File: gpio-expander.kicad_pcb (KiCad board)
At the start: 2 copper layers, 59 x 33.4 mm, 5 parts, among them U1 TPS4H160AQPWPRQ1, U2 TPS4H160AQPWPRQ1, U3 TPS4H160AQPWPRQ1, U4 TPS4H160AQPWPRQ1, U5 MCP23017T-E_SO

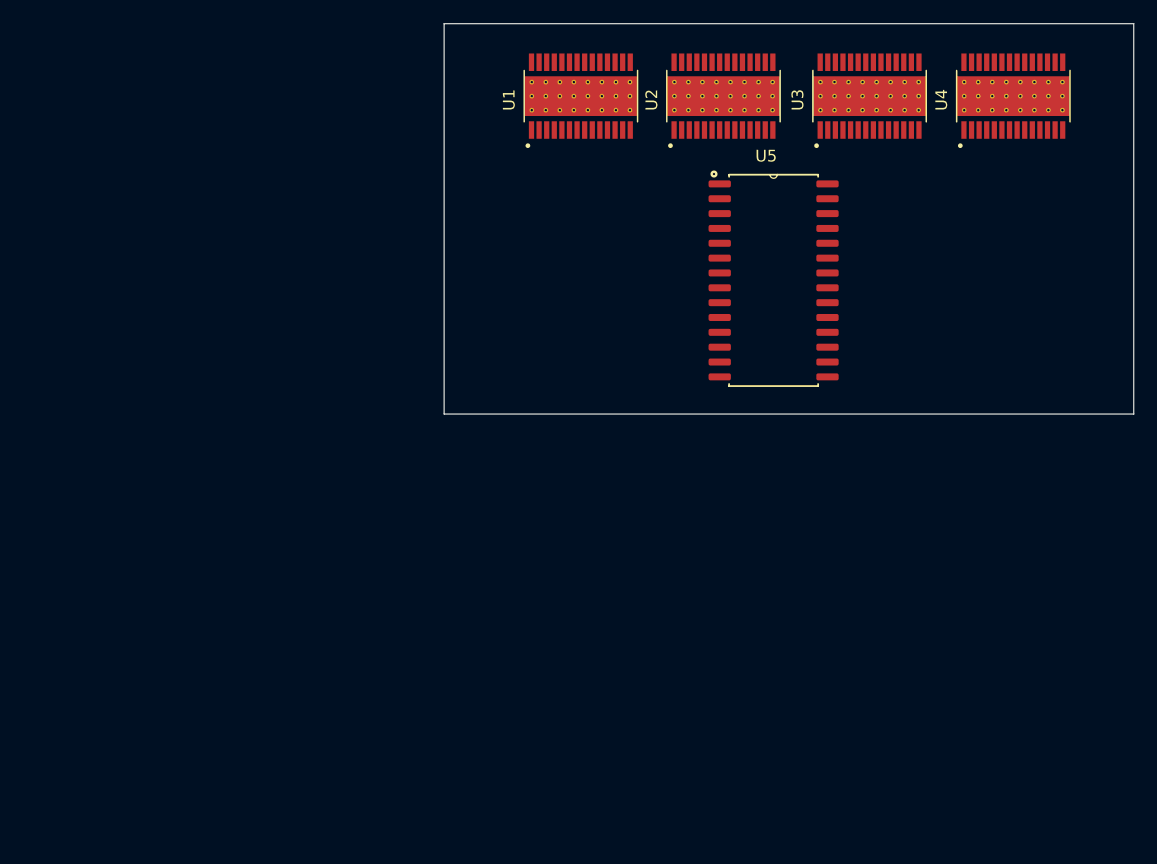
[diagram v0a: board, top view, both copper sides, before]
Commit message: first pcb revision
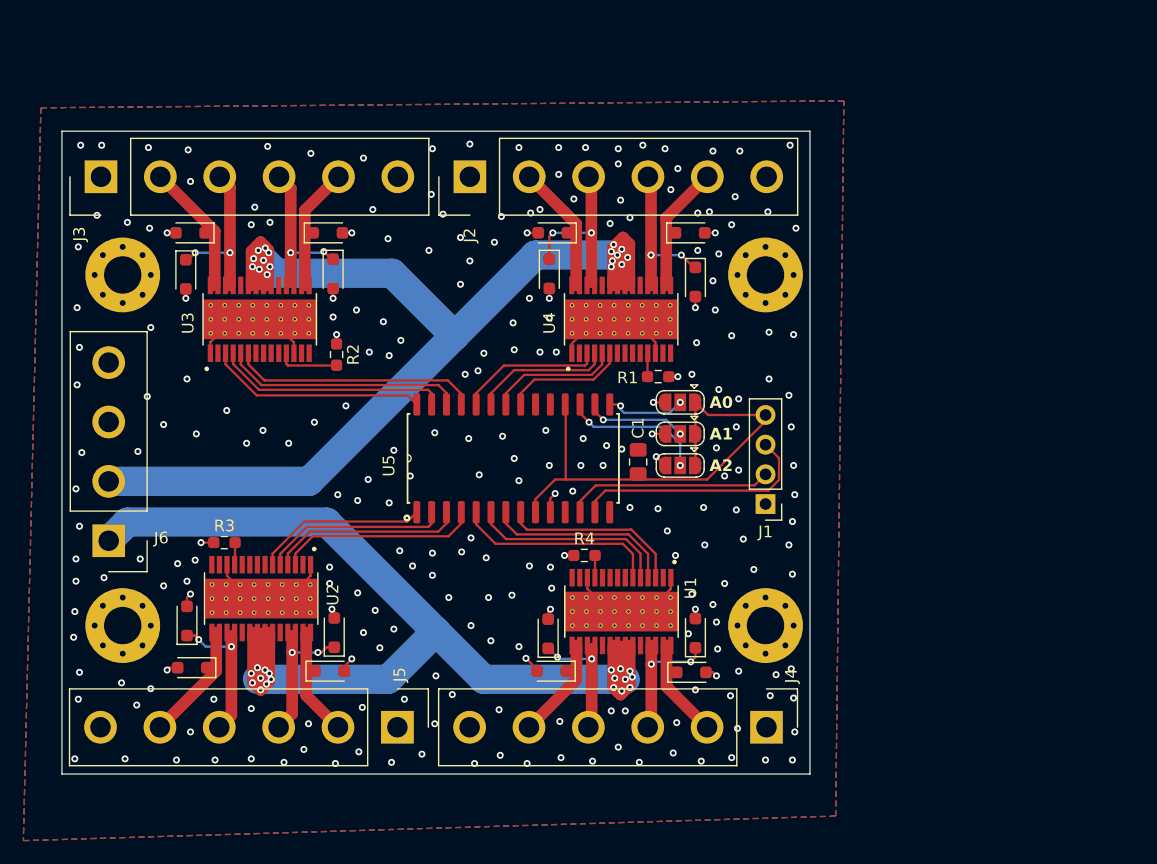
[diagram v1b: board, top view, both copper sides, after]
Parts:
- added C1: C, Capacitor_SMD:C_0805_2012Metric_Pad1.18x1.45mm_HandSolder, F.Cu at (119.1, 81.0)
- added D1: 60V 1A, Diode_SMD:D_SOD-323_HandSoldering, F.Cu at (80.8, 61.4)
- added D10: 60V 1A, Diode_SMD:D_SOD-323_HandSoldering, F.Cu at (124.0, 95.7)
- added D11: 60V 1A, Diode_SMD:D_SOD-323_HandSoldering, F.Cu at (111.4, 95.7)
- added D12: 60V 1A, Diode_SMD:D_SOD-323_HandSoldering, F.Cu at (111.7, 98.9)
- added D13: 60V 1A, Diode_SMD:D_SOD-323_HandSoldering, F.Cu at (92.7, 98.9)
- added D14: 60V 1A, Diode_SMD:D_SOD-323_HandSoldering, F.Cu at (93.1, 95.6)
- added D15: 60V 1A, Diode_SMD:D_SOD-323_HandSoldering, F.Cu at (80.5, 94.6)
- added D16: 60V 1A, Diode_SMD:D_SOD-323_HandSoldering, F.Cu at (81.0, 98.6)
- added D2: 60V 1A, Diode_SMD:D_SOD-323_HandSoldering, F.Cu at (80.4, 65.0)
- added D3: 60V 1A, Diode_SMD:D_SOD-323_HandSoldering, F.Cu at (93.0, 64.9)
- added D4: 60V 1A, Diode_SMD:D_SOD-323_HandSoldering, F.Cu at (92.5, 61.4)
- added D5: 60V 1A, Diode_SMD:D_SOD-323_HandSoldering, F.Cu at (123.5, 61.4)
- added D6: 60V 1A, Diode_SMD:D_SOD-323_HandSoldering, F.Cu at (124.0, 65.6)
- added D7: 60V 1A, Diode_SMD:D_SOD-323_HandSoldering, F.Cu at (111.5, 64.9)
- added D8: 60V 1A, Diode_SMD:D_SOD-323_HandSoldering, F.Cu at (111.8, 61.4)
- added D9: 60V 1A, Diode_SMD:D_SOD-323_HandSoldering, F.Cu at (123.7, 99.0)
- added H1: MountingHole_Pad, MountingHole:MountingHole_3.2mm_M3_Pad_Via, F.Cu at (75.0, 65.0)
- added H2: MountingHole_Pad, MountingHole:MountingHole_3.2mm_M3_Pad_Via, F.Cu at (130.0, 65.0)
- added H3: MountingHole_Pad, MountingHole:MountingHole_3.2mm_M3_Pad_Via, F.Cu at (130.0, 95.0)
- added H4: MountingHole_Pad, MountingHole:MountingHole_3.2mm_M3_Pad_Via, F.Cu at (75.0, 95.0)
- added J1: Conn_01x04, Connector_PinHeader_2.54mm:PinHeader_1x04_P2.54mm_Vertical, F.Cu at (130.0, 84.6)
- added J2: Conn_01x06, Connector_Samtec_HPM_THT:Samtec_HPM-06-05-x-S_Straight_1x06_Pitch5.08mm, F.Cu at (104.7, 56.6)
- added J3: Conn_01x06, Connector_Samtec_HPM_THT:Samtec_HPM-06-05-x-S_Straight_1x06_Pitch5.08mm, F.Cu at (73.1, 56.6)
- added J4: Conn_01x06, Connector_Samtec_HPM_THT:Samtec_HPM-06-05-x-S_Straight_1x06_Pitch5.08mm, F.Cu at (130.1, 103.7)
- added J5: Conn_01x06, Connector_Samtec_HPM_THT:Samtec_HPM-06-05-x-S_Straight_1x06_Pitch5.08mm, F.Cu at (98.5, 103.7)
- added J6: Conn_01x04, Connector_Samtec_HPM_THT:Samtec_HPM-04-05-x-S_Straight_1x04_Pitch5.08mm, F.Cu at (73.8, 87.7)
- added JP1: SolderJumper_3_Open, Jumper:SolderJumper-3_P1.3mm_Open_RoundedPad1.0x1.5mm, F.Cu at (122.7, 75.9)
- added JP2: SolderJumper_3_Open, Jumper:SolderJumper-3_P1.3mm_Open_RoundedPad1.0x1.5mm, F.Cu at (122.7, 78.6)
- added JP3: SolderJumper_3_Open, Jumper:SolderJumper-3_P1.3mm_Open_RoundedPad1.0x1.5mm, F.Cu at (122.7, 81.3)
- added R1: R, Resistor_SMD:R_0603_1608Metric_Pad0.98x0.95mm_HandSolder, F.Cu at (120.8, 73.7)
- added R2: R, Resistor_SMD:R_0603_1608Metric_Pad0.98x0.95mm_HandSolder, F.Cu at (93.3, 71.8)
- added R3: R, Resistor_SMD:R_0603_1608Metric_Pad0.98x0.95mm_HandSolder, F.Cu at (83.7, 87.9)
- added R4: R, Resistor_SMD:R_0603_1608Metric_Pad0.98x0.95mm_HandSolder, F.Cu at (114.5, 89.0)
- moved U2 58.4 mm to (86.8, 92.7), turned to -90 degrees
- moved U3 55.6 mm to (86.7, 68.8)
- moved U1 44.2 mm to (117.7, 93.8), turned to -90 degrees
- moved U4 38.6 mm to (117.7, 68.8)
- moved U5 27.0 mm to (108.4, 80.7), turned to 90 degrees
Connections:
- U1 pad 1: Net-(U1-GND-Pad1) -> GND
- U1 pad 11: unconnected-(U1-CL-Pad11) -> Net-(U1-CL)
- U1 pad 12: Net-(U1-GND-Pad1) -> GND
- U1 pad 20: Net-(U1-VS-Pad20) -> +24V
- U1 pad 21: Net-(U1-VS-Pad20) -> +24V
- U1 pad 22: Net-(U1-VS-Pad20) -> +24V
- U1 pad 23: Net-(U1-VS-Pad20) -> +24V
- U1 pad 29: Net-(U1-EXP-Pad29) -> GND
- U1 pad 30: Net-(U1-EXP-Pad29) -> GND
- U1 pad 31: Net-(U1-EXP-Pad29) -> GND
- U1 pad 32: Net-(U1-EXP-Pad29) -> GND
- U1 pad 33: Net-(U1-EXP-Pad29) -> GND
- U1 pad 34: Net-(U1-EXP-Pad29) -> GND
- U1 pad 35: Net-(U1-EXP-Pad29) -> GND
- U1 pad 36: Net-(U1-EXP-Pad29) -> GND
- U1 pad 37: Net-(U1-EXP-Pad29) -> GND
- U1 pad 38: Net-(U1-EXP-Pad29) -> GND
- U1 pad 39: Net-(U1-EXP-Pad29) -> GND
- U1 pad 40: Net-(U1-EXP-Pad29) -> GND
- U1 pad 41: Net-(U1-EXP-Pad29) -> GND
- U1 pad 42: Net-(U1-EXP-Pad29) -> GND
- U1 pad 43: Net-(U1-EXP-Pad29) -> GND
- U1 pad 44: Net-(U1-EXP-Pad29) -> GND
- U1 pad 45: Net-(U1-EXP-Pad29) -> GND
- U1 pad 46: Net-(U1-EXP-Pad29) -> GND
- U1 pad 47: Net-(U1-EXP-Pad29) -> GND
- U1 pad 48: Net-(U1-EXP-Pad29) -> GND
- U1 pad 49: Net-(U1-EXP-Pad29) -> GND
- U1 pad 50: Net-(U1-EXP-Pad29) -> GND
- U1 pad 51: Net-(U1-EXP-Pad29) -> GND
- U1 pad 52: Net-(U1-EXP-Pad29) -> GND
- U1 pad 53: Net-(U1-EXP-Pad29) -> GND
- U2 pad 1: Net-(U2-GND-Pad1) -> GND
- U2 pad 11: unconnected-(U2-CL-Pad11) -> Net-(U2-CL)
- U2 pad 12: Net-(U2-GND-Pad1) -> GND
- U2 pad 20: Net-(U2-VS-Pad20) -> +24V
- U2 pad 21: Net-(U2-VS-Pad20) -> +24V
- U2 pad 22: Net-(U2-VS-Pad20) -> +24V
- U2 pad 23: Net-(U2-VS-Pad20) -> +24V
- U2 pad 29: Net-(U2-EXP-Pad29) -> GND
- U2 pad 30: Net-(U2-EXP-Pad29) -> GND
- U2 pad 31: Net-(U2-EXP-Pad29) -> GND
- U2 pad 32: Net-(U2-EXP-Pad29) -> GND
- U2 pad 33: Net-(U2-EXP-Pad29) -> GND
- U2 pad 34: Net-(U2-EXP-Pad29) -> GND
- U2 pad 35: Net-(U2-EXP-Pad29) -> GND
- U2 pad 36: Net-(U2-EXP-Pad29) -> GND
- U2 pad 37: Net-(U2-EXP-Pad29) -> GND
- U2 pad 38: Net-(U2-EXP-Pad29) -> GND
- U2 pad 39: Net-(U2-EXP-Pad29) -> GND
- U2 pad 40: Net-(U2-EXP-Pad29) -> GND
- U2 pad 41: Net-(U2-EXP-Pad29) -> GND
- U2 pad 42: Net-(U2-EXP-Pad29) -> GND
- U2 pad 43: Net-(U2-EXP-Pad29) -> GND
- U2 pad 44: Net-(U2-EXP-Pad29) -> GND
- U2 pad 45: Net-(U2-EXP-Pad29) -> GND
- U2 pad 46: Net-(U2-EXP-Pad29) -> GND
- U2 pad 47: Net-(U2-EXP-Pad29) -> GND
- U2 pad 48: Net-(U2-EXP-Pad29) -> GND
- U2 pad 49: Net-(U2-EXP-Pad29) -> GND
- U2 pad 50: Net-(U2-EXP-Pad29) -> GND
- U2 pad 51: Net-(U2-EXP-Pad29) -> GND
- U2 pad 52: Net-(U2-EXP-Pad29) -> GND
- U2 pad 53: Net-(U2-EXP-Pad29) -> GND
- U3 pad 1: Net-(U3-GND-Pad1) -> GND
- U3 pad 11: unconnected-(U3-CL-Pad11) -> Net-(U3-CL)
- U3 pad 12: Net-(U3-GND-Pad1) -> GND
- U3 pad 20: Net-(U3-VS-Pad20) -> +24V
- U3 pad 21: Net-(U3-VS-Pad20) -> +24V
- U3 pad 22: Net-(U3-VS-Pad20) -> +24V
- U3 pad 23: Net-(U3-VS-Pad20) -> +24V
- U3 pad 29: Net-(U3-EXP-Pad29) -> GND
- U3 pad 30: Net-(U3-EXP-Pad29) -> GND
- U3 pad 31: Net-(U3-EXP-Pad29) -> GND
- U3 pad 32: Net-(U3-EXP-Pad29) -> GND
- U3 pad 33: Net-(U3-EXP-Pad29) -> GND
- U3 pad 34: Net-(U3-EXP-Pad29) -> GND
- U3 pad 35: Net-(U3-EXP-Pad29) -> GND
- U3 pad 36: Net-(U3-EXP-Pad29) -> GND
- U3 pad 37: Net-(U3-EXP-Pad29) -> GND
- U3 pad 38: Net-(U3-EXP-Pad29) -> GND
- U3 pad 39: Net-(U3-EXP-Pad29) -> GND
- U3 pad 40: Net-(U3-EXP-Pad29) -> GND
- U3 pad 41: Net-(U3-EXP-Pad29) -> GND
- U3 pad 42: Net-(U3-EXP-Pad29) -> GND
- U3 pad 43: Net-(U3-EXP-Pad29) -> GND
- U3 pad 44: Net-(U3-EXP-Pad29) -> GND
- U3 pad 45: Net-(U3-EXP-Pad29) -> GND
- U3 pad 46: Net-(U3-EXP-Pad29) -> GND
- U3 pad 47: Net-(U3-EXP-Pad29) -> GND
- U3 pad 48: Net-(U3-EXP-Pad29) -> GND
- U3 pad 49: Net-(U3-EXP-Pad29) -> GND
- U3 pad 50: Net-(U3-EXP-Pad29) -> GND
- U3 pad 51: Net-(U3-EXP-Pad29) -> GND
- U3 pad 52: Net-(U3-EXP-Pad29) -> GND
- U3 pad 53: Net-(U3-EXP-Pad29) -> GND
- U4 pad 1: Net-(U4-GND-Pad1) -> GND
- U4 pad 11: unconnected-(U4-CL-Pad11) -> Net-(U4-CL)
- U4 pad 12: Net-(U4-GND-Pad1) -> GND
- U4 pad 20: Net-(U4-VS-Pad20) -> +24V
- U4 pad 21: Net-(U4-VS-Pad20) -> +24V
- U4 pad 22: Net-(U4-VS-Pad20) -> +24V
- U4 pad 23: Net-(U4-VS-Pad20) -> +24V
- U4 pad 29: Net-(U4-EXP-Pad29) -> GND
- U4 pad 30: Net-(U4-EXP-Pad29) -> GND
- U4 pad 31: Net-(U4-EXP-Pad29) -> GND
- U4 pad 32: Net-(U4-EXP-Pad29) -> GND
- U4 pad 33: Net-(U4-EXP-Pad29) -> GND
- U4 pad 34: Net-(U4-EXP-Pad29) -> GND
- U4 pad 35: Net-(U4-EXP-Pad29) -> GND
- U4 pad 36: Net-(U4-EXP-Pad29) -> GND
- U4 pad 37: Net-(U4-EXP-Pad29) -> GND
- U4 pad 38: Net-(U4-EXP-Pad29) -> GND
- U4 pad 39: Net-(U4-EXP-Pad29) -> GND
- U4 pad 40: Net-(U4-EXP-Pad29) -> GND
- U4 pad 41: Net-(U4-EXP-Pad29) -> GND
- U4 pad 42: Net-(U4-EXP-Pad29) -> GND
- U4 pad 43: Net-(U4-EXP-Pad29) -> GND
- U4 pad 44: Net-(U4-EXP-Pad29) -> GND
- U4 pad 45: Net-(U4-EXP-Pad29) -> GND
- U4 pad 46: Net-(U4-EXP-Pad29) -> GND
- U4 pad 47: Net-(U4-EXP-Pad29) -> GND
- U4 pad 48: Net-(U4-EXP-Pad29) -> GND
- U4 pad 49: Net-(U4-EXP-Pad29) -> GND
- U4 pad 50: Net-(U4-EXP-Pad29) -> GND
- U4 pad 51: Net-(U4-EXP-Pad29) -> GND
- U4 pad 52: Net-(U4-EXP-Pad29) -> GND
- U4 pad 53: Net-(U4-EXP-Pad29) -> GND
- U5 pad 1: Net-(U3-IN1) -> Net-(U2-IN4)
- U5 pad 10: unconnected-(U5-VSS-Pad10) -> GND
- U5 pad 12: unconnected-(U5-SCK-Pad12) -> Net-(J1-Pin_2)
- U5 pad 13: unconnected-(U5-SDA-Pad13) -> Net-(J1-Pin_3)
- U5 pad 15: unconnected-(U5-A0-Pad15) -> Net-(JP1-C)
- U5 pad 16: unconnected-(U5-A1-Pad16) -> Net-(JP2-C)
- U5 pad 17: unconnected-(U5-A2-Pad17) -> Net-(JP3-C)
- U5 pad 18: unconnected-(U5-~{RESET}-Pad18) -> +3V3
- U5 pad 2: Net-(U3-IN2) -> Net-(U2-IN3)
- U5 pad 21: Net-(U1-IN1) -> Net-(U4-IN4)
- U5 pad 22: Net-(U1-IN2) -> Net-(U4-IN3)
- U5 pad 23: Net-(U1-IN3) -> Net-(U4-IN2)
- U5 pad 24: Net-(U1-IN4) -> Net-(U4-IN1)
- U5 pad 25: Net-(U2-IN1) -> Net-(U3-IN4)
- U5 pad 26: Net-(U2-IN2) -> Net-(U3-IN3)
- U5 pad 27: Net-(U2-IN3) -> Net-(U3-IN2)
- U5 pad 28: Net-(U2-IN4) -> Net-(U3-IN1)
- U5 pad 3: Net-(U3-IN3) -> Net-(U2-IN2)
- U5 pad 4: Net-(U3-IN4) -> Net-(U2-IN1)
- U5 pad 5: Net-(U4-IN1) -> Net-(U1-IN4)
- U5 pad 6: Net-(U4-IN2) -> Net-(U1-IN3)
- U5 pad 7: Net-(U4-IN3) -> Net-(U1-IN2)
- U5 pad 8: Net-(U4-IN4) -> Net-(U1-IN1)
- U5 pad 9: unconnected-(U5-VDD-Pad9) -> +3V3
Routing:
- net +24V: track 0.00 -> 207.2 mm, vias 0 -> 35
- net GND: track 0.00 -> 66.4 mm, vias 0 -> 251
- net +3V3: track 0.00 -> 42.4 mm
- net Net-(U3-IN4): track 0.00 -> 21.1 mm
- net Net-(J1-Pin_3): track 0.00 -> 20.9 mm
- net Net-(U3-IN3): track 0.00 -> 20.5 mm
- net Net-(U3-IN2): track 0.00 -> 19.9 mm
- net Net-(U3-IN1): track 0.00 -> 18.7 mm
- net Net-(J1-Pin_2): track 0.00 -> 17.8 mm
- net Net-(U1-IN4): track 0.00 -> 17.5 mm
- net Net-(U2-IN1): track 0.00 -> 17.2 mm
- net Net-(U1-IN3): track 0.00 -> 16.9 mm
- net Net-(U2-IN2): track 0.00 -> 16.6 mm
- net Net-(U1-IN2): track 0.00 -> 16.2 mm
- net Net-(U2-IN3): track 0.00 -> 15.9 mm
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- added copper zone on B.Cu, net GND
- added copper zone on F.Cu, net GND
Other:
- board size 59 x 33.4 mm -> 64 x 55 mm
- board text added: "A0"
- board text added: "A1"
- board text added: "A2"
